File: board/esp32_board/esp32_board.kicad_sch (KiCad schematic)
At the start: 7 parts, among them J1 Screw_Terminal_01x19, J2 Screw_Terminal_01x19, J3 Conn_01x19_Socket, J4 Conn_01x19_Pin, J5 Conn_01x19_Socket, J6 Conn_01x19_Pin, U1 ESP32-DevKitC

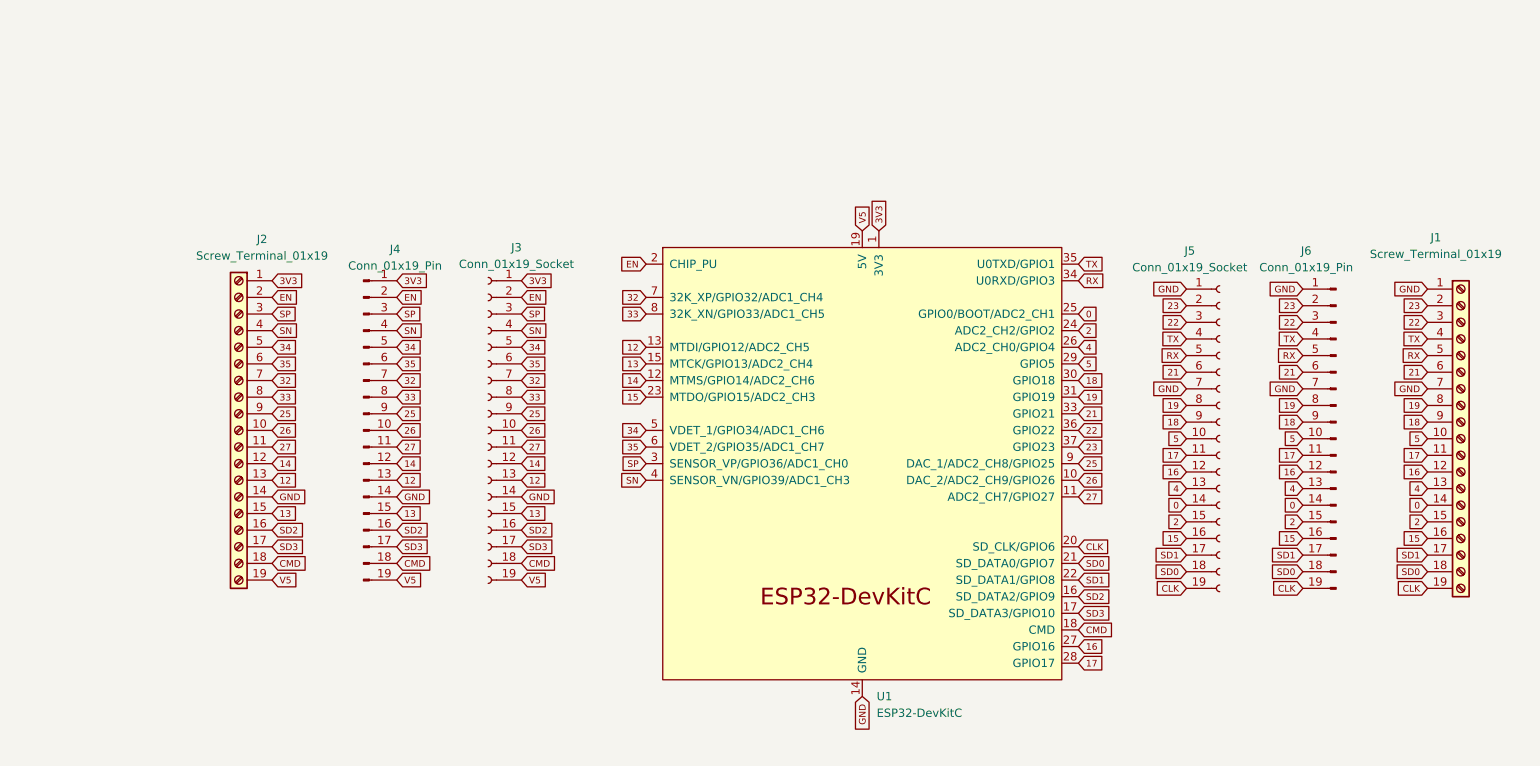
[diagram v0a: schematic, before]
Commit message: feat: Updated board and presentation
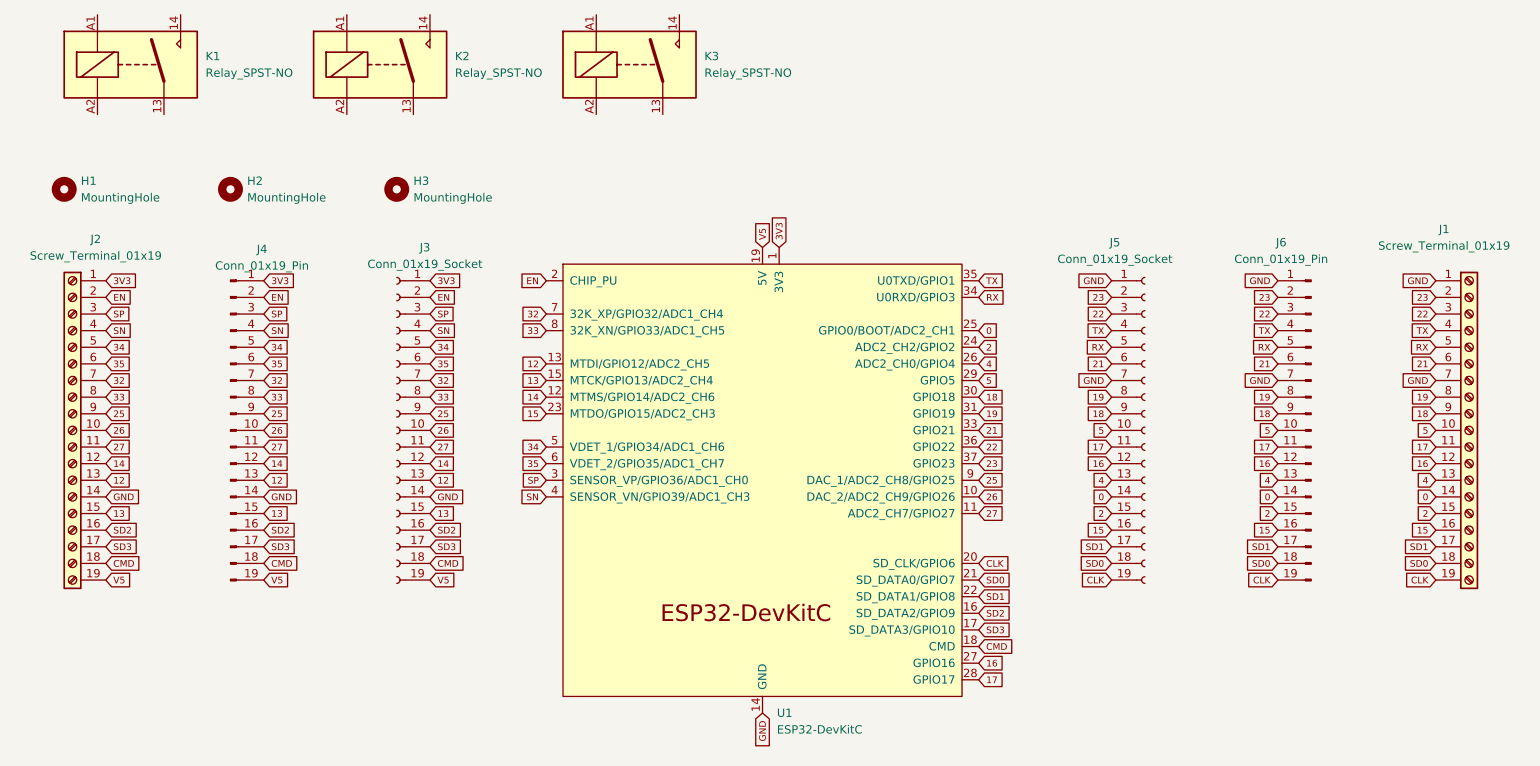
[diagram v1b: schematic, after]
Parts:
- added H1, H2, H3: MountingHole, symbol Mechanical:MountingHole
- added K1, K2, K3: Relay_SPST-NO, symbol Relay:Relay_SPST-NO
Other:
- moved on the sheet: J1, J2, J3, J4, J5, J6, U1
